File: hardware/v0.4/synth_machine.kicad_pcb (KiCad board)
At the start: 2 copper layers, 160 x 74 mm, 123 parts, among them J1 USB-C (MIDI + 5V power), J10 Pot VOL (10k lin, panel) JST-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, J15 STEMMA QT (I2C1), J16 Power switch (panel SPST) JST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, J17 Battery 1S LiPo (JST-PH, 1 = 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, J5 Speaker L (JST-PH), J6 Speaker R (JST-PH), J7 Headphones 3.5mm (CUI SJ1-351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, J8 Expansion, J9 Display (SPI1), K1 KEY C4 (direct D10) JST-XH, K10 A4 [c2 r2] JST-XH, K11 A#4 [c1 r1] JST-XH, K12 B4 [c1 r2] JST-XH, K13 C5 [c0 r2] JST-XH, K14 BTN1 [c0 r0] JST-XH, K15 BTN2 [c0 r1] JST-XH, K16 BTN3 [c1 r0] JST-XH, K17 BTN4 [c2 r0] JST-XH, K18 BTN5 [c3 r0] JST-XH, K19 BTN6 [c4 r0] JST-XH, K2 C#4 [c5 r0] JST-XH, K3 D4 [c5 r1] JST-XH, K4 D#4 [c4 r1] JST-XH, K5 E4 [c5 r2] JST-XH, K6 F4 [c4 r2] JST-XH, K7 F#4 [c3 r1] JST-XH, K8 G4 [c3 r2] JST-XH, K9 G#4 [c2 r1] JST-XH, Q1 2N7002, Q2 2N7002, U1 Daisy Seed / Seed3, U2 TPA6138A2PWR, U3 MAX98306ETD+T, U4 USBLC6-2SC6, U5 BQ24074RGTR, U6 TPS61023DRLR, U7 AP7361C-33E-13

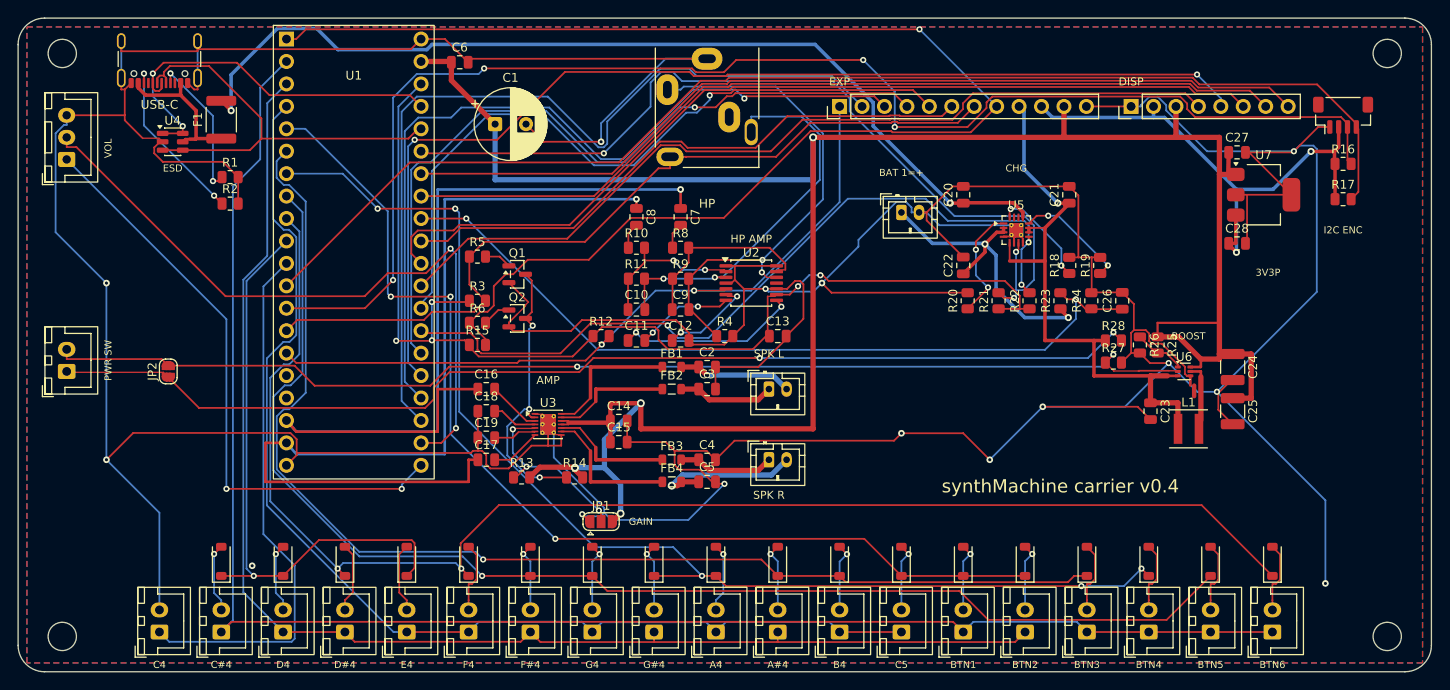
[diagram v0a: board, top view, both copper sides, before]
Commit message: Carrier v0.4: JP1 (amp gain) moved to the open area right of the speaker connectors
4 mm or more clear on every side for soldering; it was 2 mm from the key
diode row. DRC 0 unconnected, ERC clean.

Co-Authored-By: Claude Fable 5.1 <noreply@anthropic.com>
Claude-Session: https://claude.ai/code/session_019ZDGV5fm4G7LwUwRWHEiwx
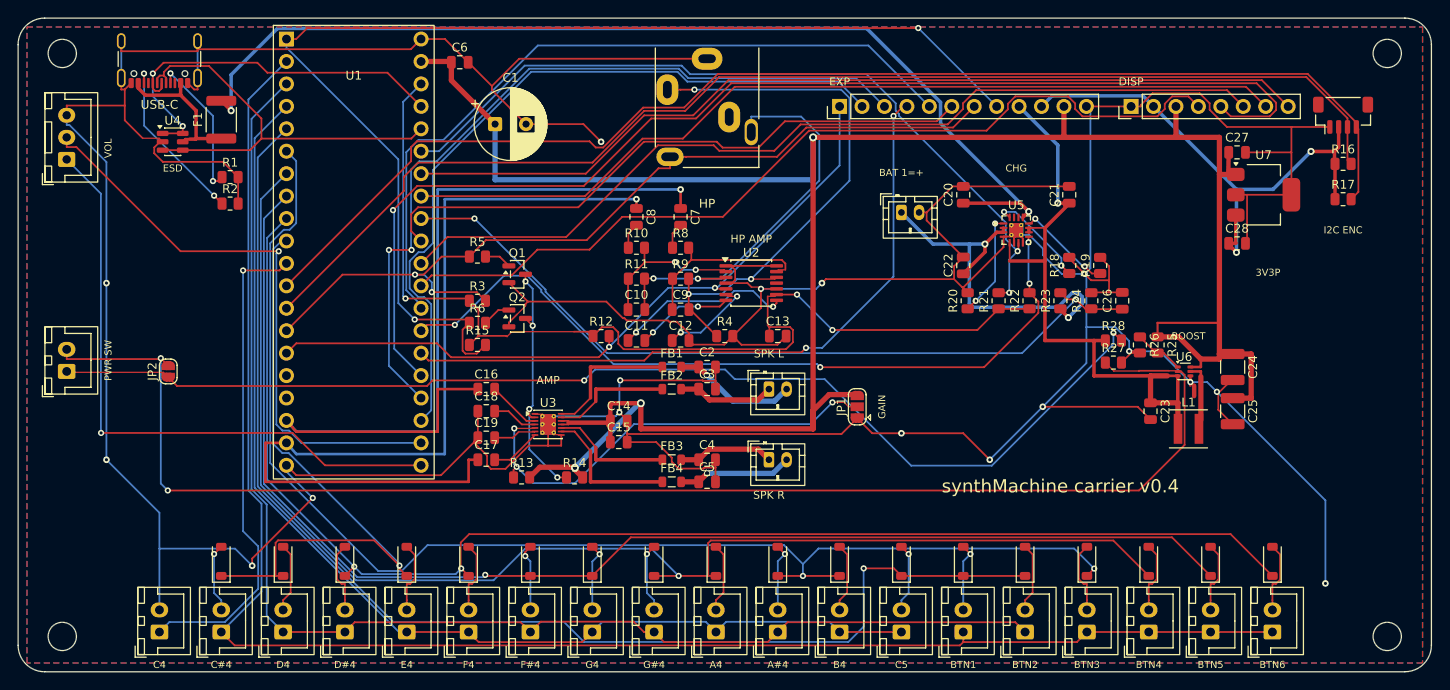
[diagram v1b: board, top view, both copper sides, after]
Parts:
- moved JP1 31.8 mm to (95.0, 44.0), turned to 90 degrees
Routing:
- net GND: track 737.2 -> 680.7 mm, vias 15 -> 17
- net BOOST_EN: track 132.2 -> 163.0 mm
- net AMP_GAIN: track 21.1 -> 51.5 mm
- net COL0: track 119.2 -> 143.7 mm, vias 3 -> 1
- net MUTE: track 159.0 -> 135.4 mm, vias 1 -> 2
- net I2C_SDA: track 157.9 -> 139.2 mm, vias 4 -> 0
- net COL2: track 136.8 -> 153.4 mm, vias 5 -> 1
- net POT_VOL: track 79.0 -> 67.0 mm, vias 2 -> 1
- net COL1: track 137.2 -> 149.0 mm, vias 1 -> 2
- net EXP_A1: track 98.0 -> 86.5 mm
- net USB_PGOOD: track 100.1 -> 89.3 mm, vias 3 -> 2
- net SPI_MOSI: track 124.4 -> 134.7 mm, vias 2 -> 1
- net EXP_A4: track 86.4 -> 77.9 mm, vias 1 -> 2
- net VBAT: track 35.0 -> 43.4 mm
- net VUSB: track 108.8 -> 116.8 mm
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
